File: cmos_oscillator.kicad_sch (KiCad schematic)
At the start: 8 parts, among them X1 YC24.576MUBCE2O

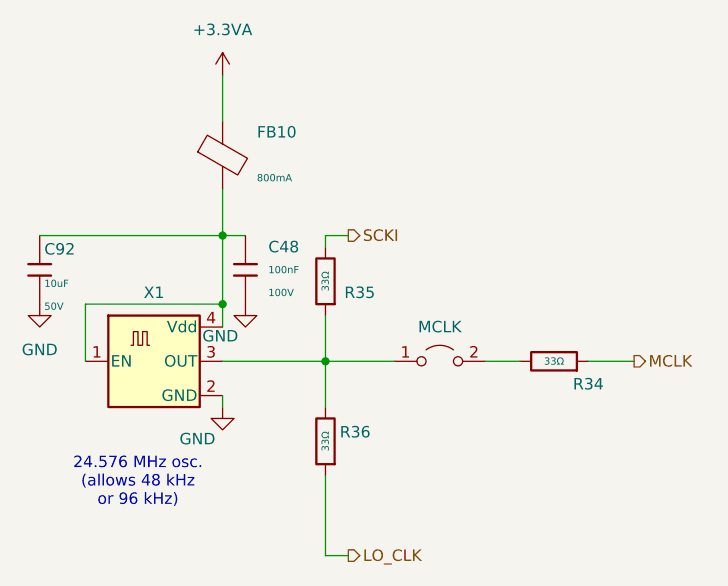
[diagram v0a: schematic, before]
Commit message: Added CJC5340
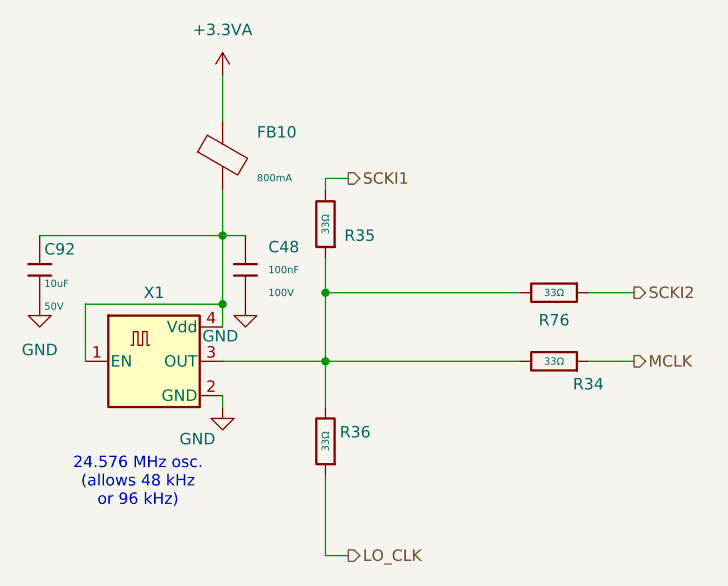
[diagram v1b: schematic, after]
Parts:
- removed JP5: MCLK, Jumper:SolderJumper-2_P1.3mm_Open_RoundedPad1.0x1.5mm, symbol Jumper:Jumper_2_Open
- added R76: 33Ω, PCM_JLCPCB:R_0805, symbol PCM_JLCPCB-Resistors:0805,33Ω
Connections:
- net at R35.1, R36.2, X1.3 (OUT): now also R34.2, R76.2
- net SCKI renamed SCKI1
- new net SCKI2: R76.1
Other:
- moved on the sheet: R35
